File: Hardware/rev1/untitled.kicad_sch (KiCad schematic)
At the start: 16 parts, among them J2 USB_C_Receptacle_USB2.0_14P, J3 Screw_Terminal_01x02, U2 HT75xx-1-SOT89

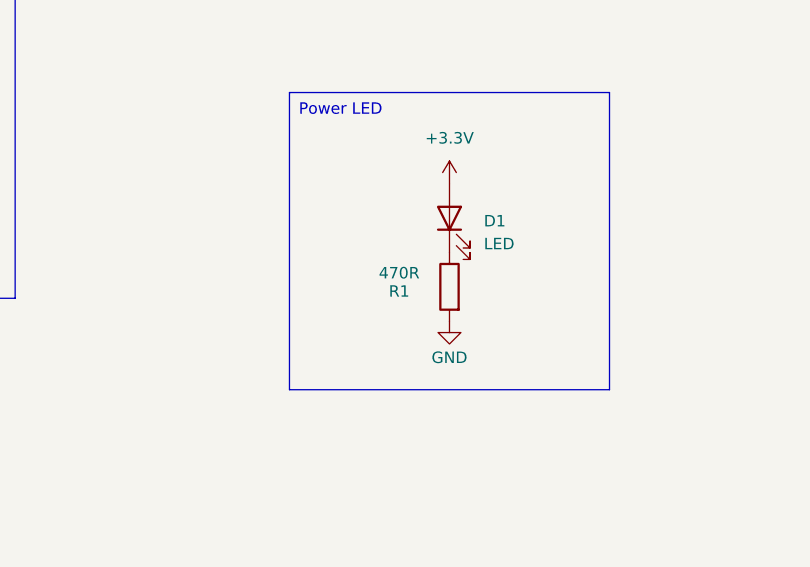
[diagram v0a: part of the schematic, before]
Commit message: Revert "Merge remote-tracking branch 'origin/dev'"
This reverts commit 9d6b38d1428df59ab2602e839e1db75647d3fbc2, reversing
changes made to aa461fd2fa90bcdcb689545e3dbed326723346fe.
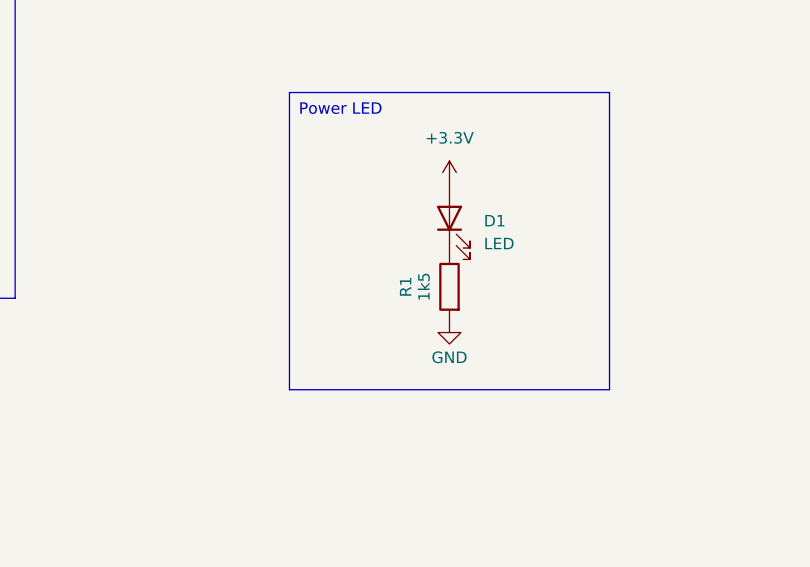
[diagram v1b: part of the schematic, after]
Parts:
- BT1: footprint Battery:BatteryHolder_Keystone_3034_1x20mm -> (none)
- C10, C8, C9: footprint Capacitor_SMD:C_0603_1608Metric -> (none)
- C7: footprint Capacitor_SMD:C_0402_1005Metric -> (none)
- D1: footprint LED_SMD:LED_0201_0603Metric -> (none)
- D2, D3: footprint Diode_SMD:D_SOD-123F -> (none)
- J2: footprint Connector_USB:USB_C_Receptacle_HRO_TYPE-C-31-M-12 -> (none)
- J3: footprint TerminalBlock:TerminalBlock_Xinya_XY308-2.54-2P_1x02_P2.54mm_Horizontal -> (none)
- NT1: footprint NetTie:NetTie-2_SMD_Pad2.0mm -> (none)
- R1: value 470R -> 1k5; footprint Resistor_SMD:R_0603_1608Metric -> Resistor_SMD:R_0402_1005Metric
- R3, R4, R5: footprint Resistor_SMD:R_0603_1608Metric -> Resistor_SMD:R_0402_1005Metric
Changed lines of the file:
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@@
 			)
 		)
-		(property "Footprint" "Resistor_SMD:R_0603_1608Metric"
+		(property "Footprint" "Resistor_SMD:R_0402_1005Metric"
 			(at 70.358 72.39 90)
 			(effects
@@
 			)
 		)
-		(property "Footprint" "LED_SMD:LED_0201_0603Metric"
+		(property "Footprint" ""
 			(at 151.13 90.17 0)
 			(effects
@@
 			)
 		)
-		(property "Footprint" "Capacitor_SMD:C_0603_1608Metric"
+		(property "Footprint" ""
 			(at 79.7052 163.83 0)
 			(effects
@@
 			)
 		)
-		(property "Footprint" "Capacitor_SMD:C_0603_1608Metric"
+		(property "Footprint" ""
 			(at 239.7252 100.33 0)
 			(effects
@@
 			)
 		)
-		(property "Footprint" "NetTie:NetTie-2_SMD_Pad2.0mm"
+		(property "Footprint" ""
 			(at 222.25 92.71 0)
 			(effects
@@
 			)
 		)
-		(property "Footprint" "Diode_SMD:D_SOD-123F"
+		(property "Footprint" ""
 			(at 50.8 135.89 0)
 			(effects
@@
 		(dnp no)
 		(property "Reference" "R1"
-			(at 145.542 98.298 0)
-			(effects
-				(font
-					(size 1.27 1.27)
-				)
-			)
-		)
-		(property "Value" "470R"
-			(at 145.542 96.266 0)
-			(effects
-				(font
-					(size 1.27 1.27)
-				)
-			)
-		)
-		(property "Footprint" "Resistor_SMD:R_0603_1608Metric"
+			(at 146.304 97.79 90)
+			(effects
+				(font
+					(size 1.27 1.27)
+				)
+			)
+		)
+		(property "Value" "1k5"
+			(at 148.336 97.79 90)
+			(effects
+				(font
+					(size 1.27 1.27)
+				)
+			)
+		)
+		(property "Footprint" "Resistor_SMD:R_0402_1005Metric"
 			(at 152.908 97.79 90)
 			(effects
@@
 			)
 		)
-		(property "Footprint" "Capacitor_SMD:C_0402_1005Metric"
+		(property "Footprint" ""
 			(at 230.8352 100.33 0)
 			(effects
@@
 			)
 		)
-		(property "Footprint" "TerminalBlock:TerminalBlock_Xinya_XY308-2.54-2P_1x02_P2.54mm_Horizontal"
+		(property "Footprint" ""
 			(at 68.58 139.7 0)
 			(effects
@@
 			)
 		)
-		(property "Footprint" "Diode_SMD:D_SOD-123F"
+		(property "Footprint" ""
 			(at 60.96 135.89 0)
 			(effects
@@
 			)
 		)
-		(property "Footprint" "Battery:BatteryHolder_Keystone_3034_1x20mm"
+		(property "Footprint" ""
 			(at 147.574 41.91 90)
 			(effects
@@
 			)
 		)
-		(property "Footprint" "Resistor_SMD:R_0603_1608Metric"
+		(property "Footprint" "Resistor_SMD:R_0402_1005Metric"
 			(at 81.28 52.578 90)
 			(effects
@@
 			)
 		)
-		(property "Footprint" "Resistor_SMD:R_0603_1608Metric"
+		(property "Footprint" "Resistor_SMD:R_0402_1005Metric"
 			(at 81.28 51.562 90)
 			(effects
@@
 			)
 		)
-		(property "Footprint" "Connector_USB:USB_C_Receptacle_HRO_TYPE-C-31-M-12"
+		(property "Footprint" ""
 			(at 55.88 60.96 0)
 			(effects
@@
 			)
 		)
-		(property "Footprint" "Capacitor_SMD:C_0603_1608Metric"
+		(property "Footprint" ""
 			(at 49.2252 163.83 0)
 			(effects
